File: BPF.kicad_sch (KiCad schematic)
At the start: 48 parts, among them Q17 BC548, Q18 BC548, Q19 BC548, Q20 BC548, Q21 BC548, Q22 BC548, Q23 BC548, Q24 BC548, Q25 BC548, Q26 BC548, Q27 BC548, Q28 BC548, Q29 BC548, Q30 BC548, Q31 BC548, Q32 BC548

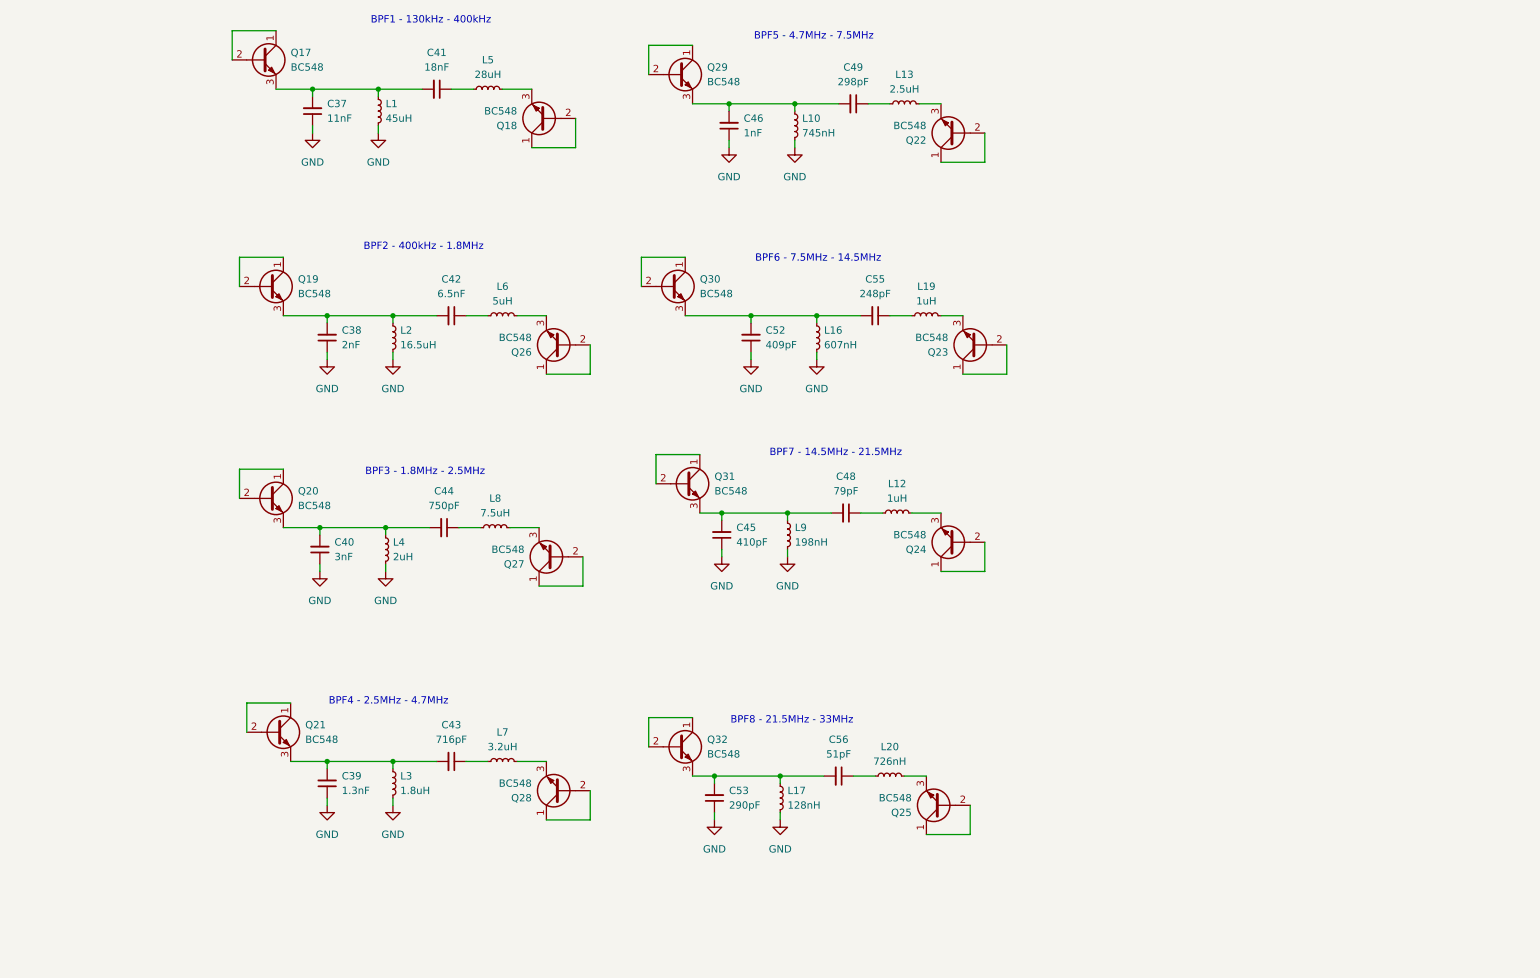
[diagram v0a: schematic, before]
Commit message: BPF Work 3
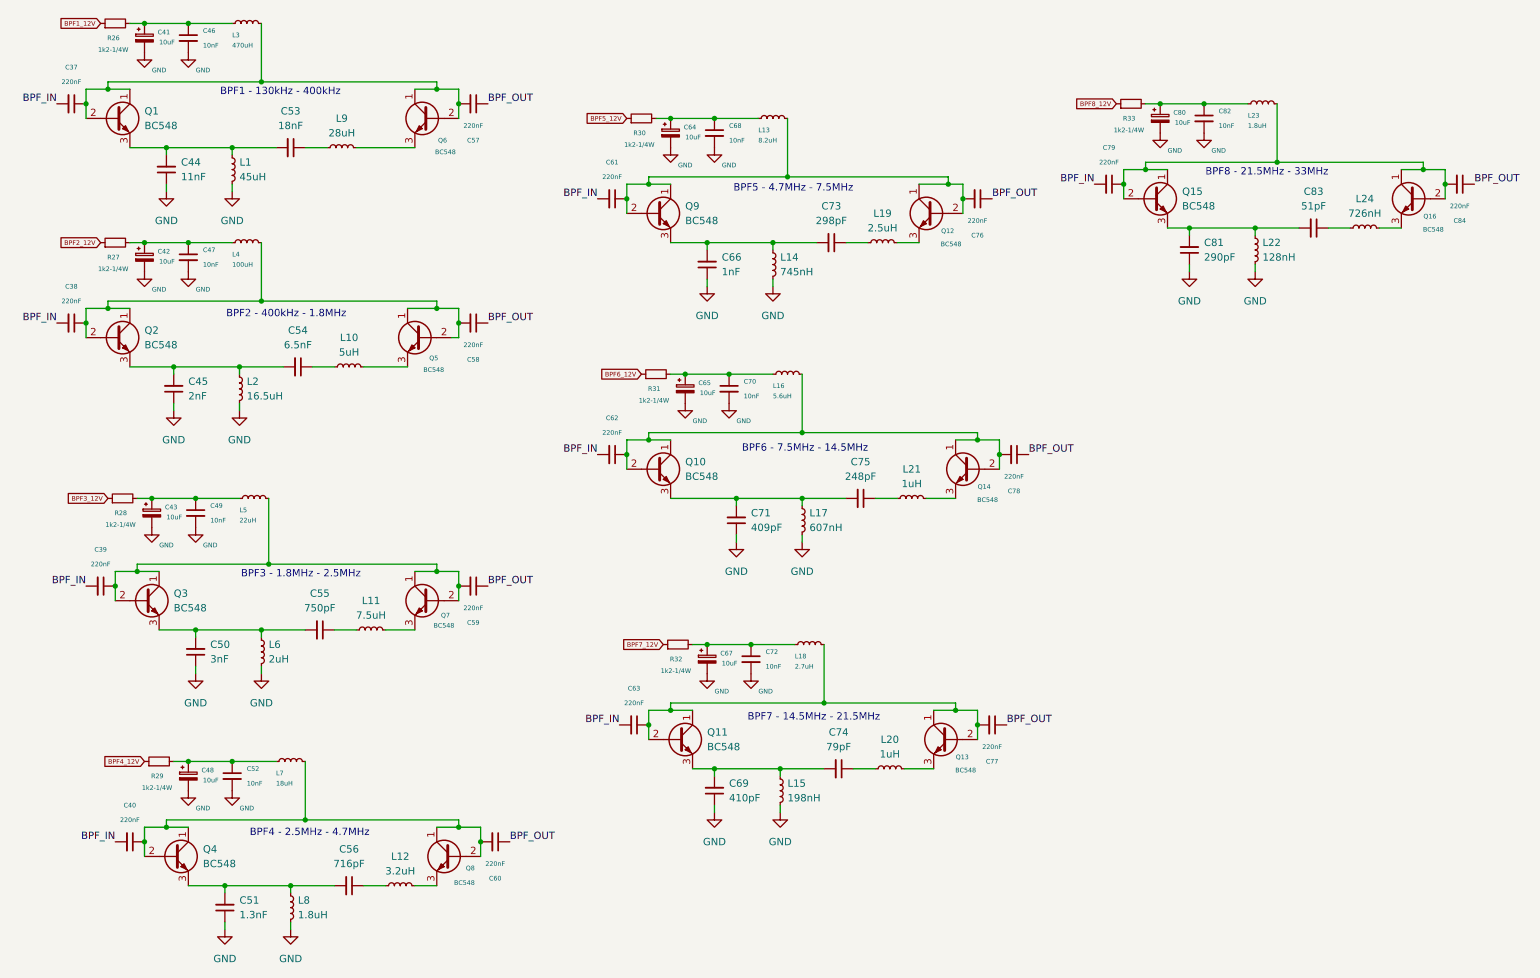
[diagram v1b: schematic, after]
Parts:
- removed Q23, Q24, Q25: BC548, Package_TO_SOT_THT:TO-92_Inline, symbol Transistor_BJT:BC548
- added C37, C38, C39, C40, C57, C58, C59, C60, C61, C62, C63, C76, C77, C78, C79, C84: 220nF, symbol Device:C_Small
- added C41, C42, C43, C48, C64, C65, C67, C80: 10uF, symbol Device:C_Polarized_Small
- added C46, C47, C49, C52, C68, C70, C72, C82: 10nF, symbol Device:C_Small
- added L13: 8.2uH, symbol Device:L_Small
- added L16: 5.6uH, symbol Device:L_Small
- added L18: 2.7uH, symbol Device:L_Small
- added L23: 1.8uH, symbol Device:L_Small
- added L3: 470uH, symbol Device:L_Small
- added L4: 100uH, symbol Device:L_Small
- added L5: 22uH, symbol Device:L_Small
- added L7: 18uH, symbol Device:L_Small
- added Q13, Q14, Q16: BC548, Package_TO_SOT_THT:TO-92_Inline, symbol Transistor_BJT:BC548
- added R26, R27, R28, R29, R30, R31, R32, R33: 1k2-1/4W, symbol Device:R_Small
- renumbered C37 to C44, C38 to C45, C40 to C50, C39 to C51, C41 to C53, C42 to C54, C44 to C55, C43 to C56, C46 to C66, C45 to C69, C52 to C71, C49 to C73, C48 to C74, C55 to C75, C53 to C81, C56 to C83, L6 to L10, L8 to L11, L7 to L12, L10 to L14, L9 to L15, L16 to L17, L13 to L19, L12 to L20, L19 to L21, L17 to L22, L20 to L24, L4 to L6, L3 to L8, L5 to L9, Q17 to Q1, Q30 to Q10, Q31 to Q11, Q22 to Q12, Q32 to Q15, Q19 to Q2, Q20 to Q3, Q21 to Q4, Q26 to Q5, Q18 to Q6, Q27 to Q7, Q28 to Q8, Q29 to Q9
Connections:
- net GND: now also C41.2, C42.2, C43.2, C46.2, C47.2, C48.2, C49.2, C52.2, C64.2, C65.2, C67.2, C68.2, C70.2, C72.2, C80.2, C82.2
- net at Q9.1 (C), Q9.2 (B): now also Q12.1 (C), Q12.2 (B), C61.1, C76.2, L13.2
- net at Q1.1 (C), Q1.2 (B): now also Q6.1 (C), Q6.2 (B), C37.1, C57.2, L3.2
- net at Q5.1 (C), Q5.2 (B): now also Q2.1 (C), Q2.2 (B), C38.1, C58.2, L4.2
- net at L21.2: now also Q14.3 (E)
- net at Q8.1 (C), Q8.2 (B): now also Q4.1 (C), Q4.2 (B), C40.1, C60.2, L7.2
- net at L24.2: now also Q16.3 (E)
- net at Q7.1 (C), Q7.2 (B): now also Q3.1 (C), Q3.2 (B), C39.1, C59.2, L5.2
- net at L20.2: now also Q13.3 (E)
- net at Q11.1 (C), Q11.2 (B): now also C63.1, C77.2, L18.2, Q13.1 (C), Q13.2 (B)
- net at Q15.1 (C), Q15.2 (B): now also C79.1, C84.2, L23.2, Q16.1 (C), Q16.2 (B)
- net at Q10.1 (C), Q10.2 (B): now also C62.1, C78.2, L16.2, Q14.1 (C), Q14.2 (B)
- new net: C65.1, C70.1, L16.1, R31.2
- new net: C64.1, C68.1, L13.1, R30.2
- new net: C41.1, C46.1, L3.1, R26.2
- new net: C67.1, C72.1, L18.1, R32.2
- new net: C43.1, C49.1, L5.1, R28.2
- new net: C42.1, C47.1, L4.1, R27.2
- new net: C48.1, C52.1, L7.1, R29.2
- new net: C80.1, C82.1, L23.1, R33.2
- new net BPF1_12V: R26.1
- new net BPF2_12V: R27.1
- new net BPF3_12V: R28.1
- new net BPF4_12V: R29.1
- new net BPF5_12V: R30.1
- new net BPF6_12V: R31.1
- new net BPF7_12V: R32.1
- new net BPF8_12V: R33.1
- new net BPF_IN: C37.2, C38.2, C39.2, C40.2, C61.2, C62.2, C63.2, C79.2
- new net BPF_OUT: C57.1, C58.1, C59.1, C60.1, C76.1, C77.1, C78.1, C84.1
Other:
- moved on the sheet: C44, C45, C50, C51, C53, C54, C55, C56, C66, C69, C71, C73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
